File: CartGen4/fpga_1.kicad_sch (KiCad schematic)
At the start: 5 parts, among them U9 LFXP2-8E-5MN132C

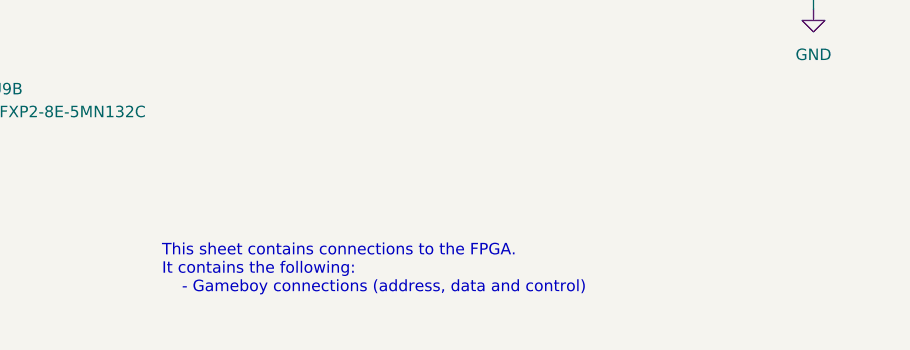
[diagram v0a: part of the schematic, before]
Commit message: Minor adjustments
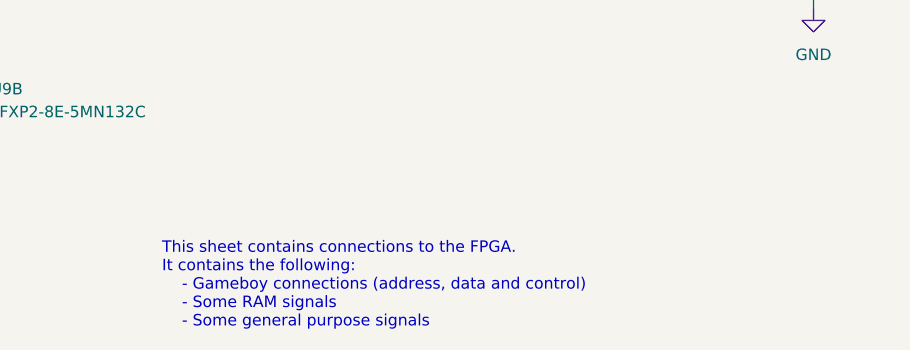
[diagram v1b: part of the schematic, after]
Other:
- note added: "This sheet contains connections to the FPGA. It contains the following: - Gameboy connections (address, data and control) - Some RAM signals - Some general purpose signals"
- note removed: "This sheet contains connections to the FPGA. It contains the following: - Gameboy connections (address, data and control)"
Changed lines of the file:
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@@
     (stroke (width 0) (type default) (color 0 0 0 0))
   )
-  (text "This sheet contains connections to the FPGA.\nIt contains the following:\n    - Gameboy connections (address, data and control)"
-    (at 179.07 173.99 0)
+  (text "This sheet contains connections to the FPGA.\nIt contains the following:\n    - Gameboy connections (address, data and control)\n    - Some RAM signals\n    - Some general purpose signals"
+    (at 179.07 177.8 0)
     (effects (font (size 1.27 1.27)) (justify left bottom))
   )
